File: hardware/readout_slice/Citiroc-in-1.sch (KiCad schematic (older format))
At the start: 6 parts

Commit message: need to fix one rescure in readout_slice
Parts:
- U?: symbol readout_slice-rescue:CITIROC1A-readout -> readout_slice-rescue:CITIROC1A-readout-readout_slice-rescue
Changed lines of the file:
@@
 $Descr A4 11693 8268
 encoding utf-8
-Sheet 7 16
+Sheet 6 16
 Title ""
 Date ""
@@
 	9450 1600 3800 1600
 $Comp
-L readout_slice-rescue:CITIROC1A-readout U?
+L readout_slice-rescue:CITIROC1A-readout-readout_slice-rescue U?
 U 3 1 60AFA4EB
 P 10100 900

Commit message: getting rid of readout_slice rescue
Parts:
- U?: symbol readout_slice-rescue:CITIROC1A-readout-readout_slice-rescue -> readout:CITIROC1A
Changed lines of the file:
@@
 	9450 1600 3800 1600
 $Comp
-L readout_slice-rescue:CITIROC1A-readout-readout_slice-rescue U?
+L readout:CITIROC1A U?
 U 3 1 60AFA4EB
 P 10100 900

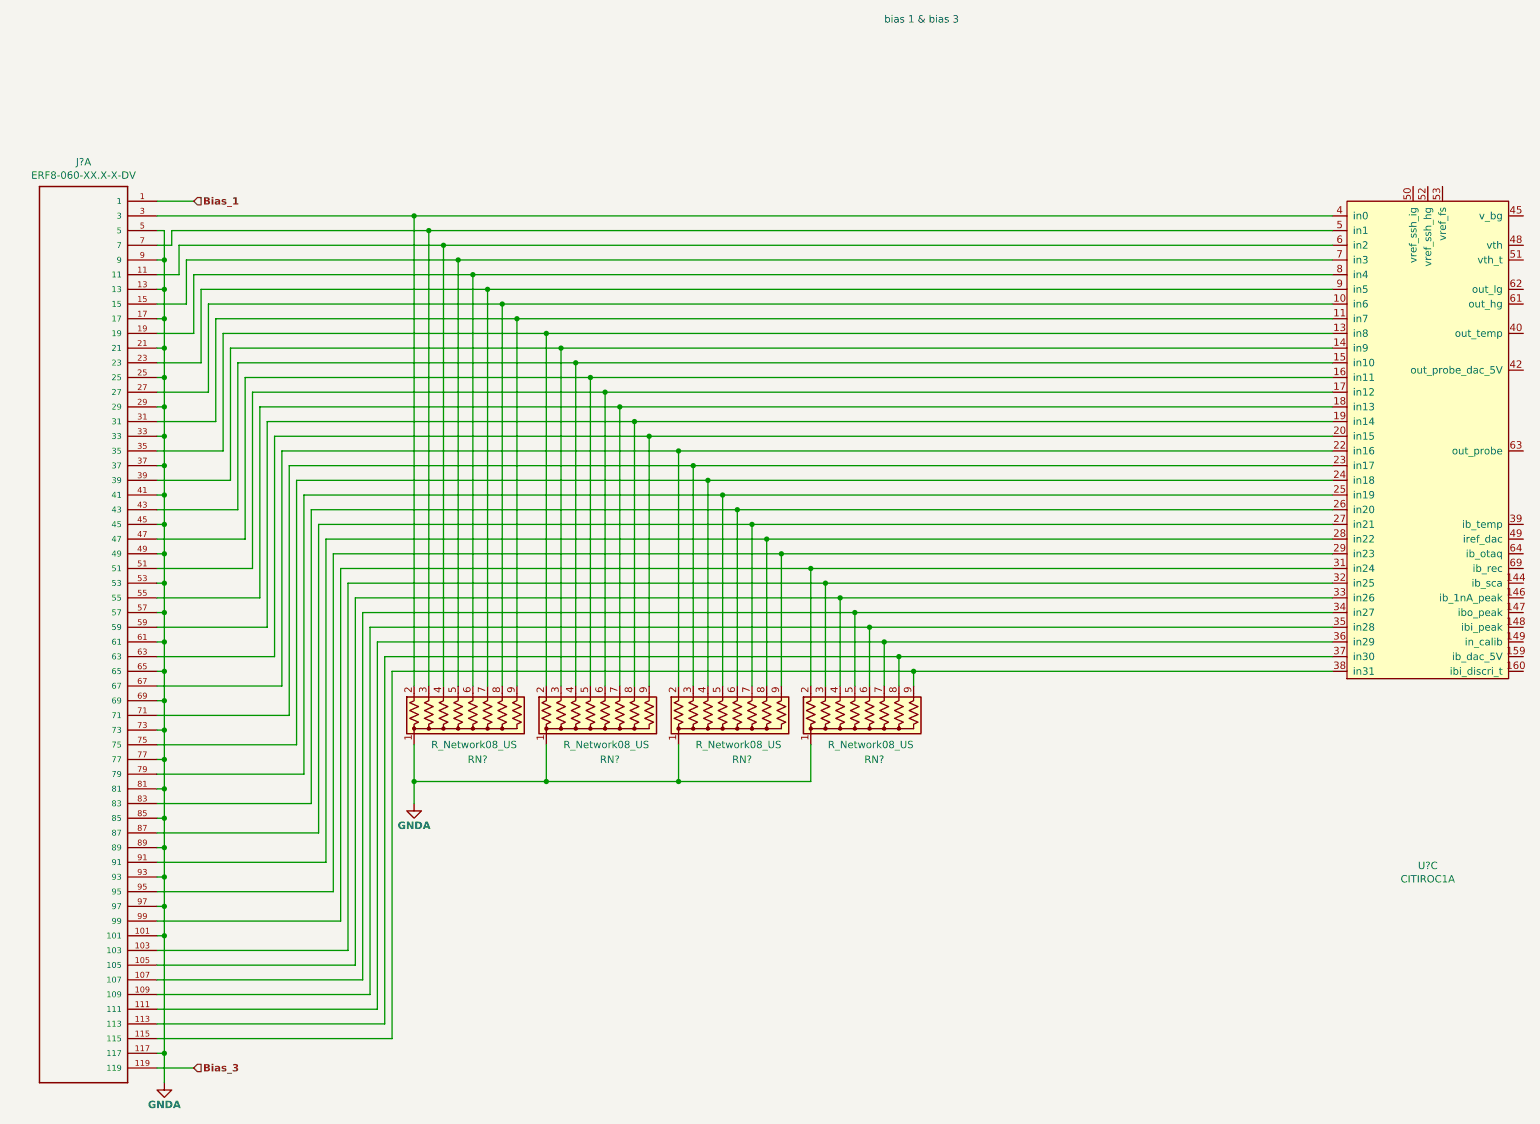
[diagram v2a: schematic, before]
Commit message: more progress on readout_slice
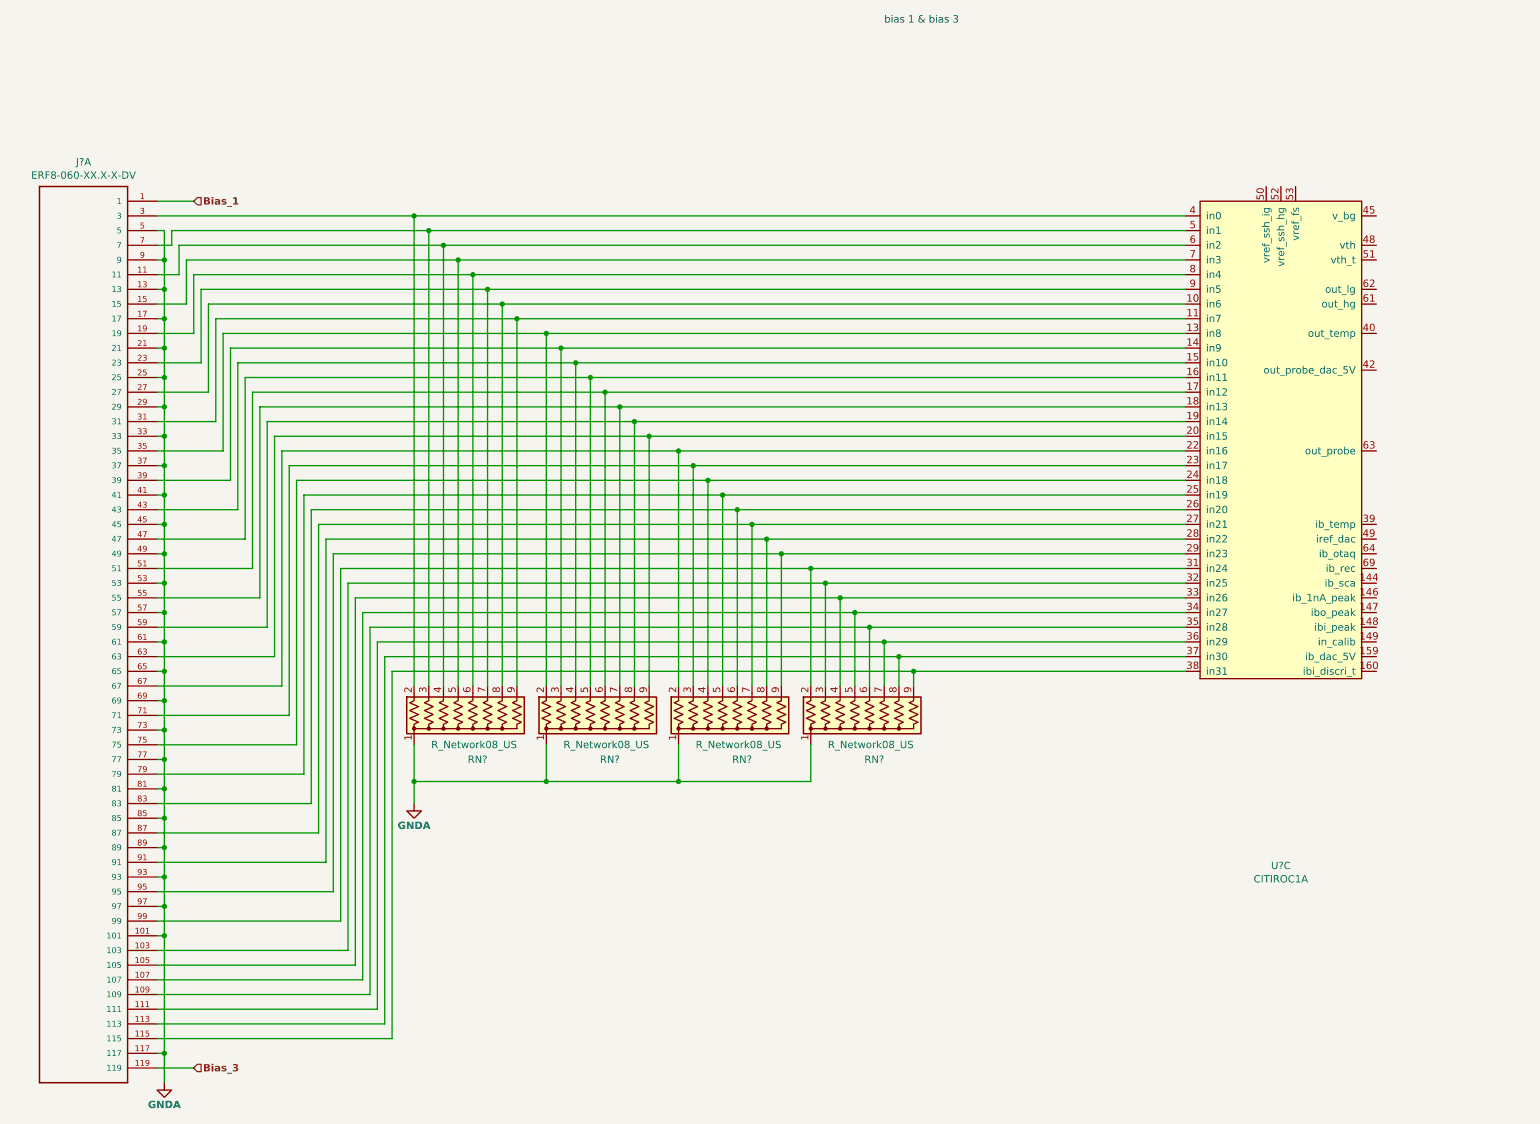
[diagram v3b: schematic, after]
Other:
- moved on the sheet: U?C
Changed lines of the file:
@@
 	1700 6800 1450 6800
 Wire Wire Line
-	3700 1500 9450 1500
+	3700 1500 8450 1500
 Wire Wire Line
-	9450 1400 3600 1400
+	8450 1400 3600 1400
 Wire Wire Line
-	3500 1300 9450 1300
+	3500 1300 8450 1300
 Wire Wire Line
-	9450 1200 3400 1200
+	8450 1200 3400 1200
 Wire Wire Line
-	3300 1100 9450 1100
+	3300 1100 8450 1100
 Wire Wire Line
-	9450 1000 3200 1000
+	8450 1000 3200 1000
 Wire Wire Line
-	6600 4100 9450 4100
+	6600 4100 8450 4100
 Wire Wire Line
-	6500 4000 9450 4000
+	6500 4000 8450 4000
 Wire Wire Line
-	6400 3900 9450 3900
+	6400 3900 8450 3900
 Wire Wire Line
-	6300 3800 9450 3800
+	6300 3800 8450 3800
 Wire Wire Line
-	6200 3700 9450 3700
+	6200 3700 8450 3700
 Wire Wire Line
-	9450 3600 6100 3600
+	8450 3600 6100 3600
 Wire Wire Line
-	9450 3500 6000 3500
+	8450 3500 6000 3500
 Wire Wire Line
-	5900 3400 9450 3400
+	5900 3400 8450 3400
 Wire Wire Line
-	9450 3300 5700 3300
+	8450 3300 5700 3300
 Wire Wire Line
-	5600 3200 9450 3200
+	5600 3200 8450 3200
 Wire Wire Line
-	9450 3100 5500 3100
+	8450 3100 5500 3100
 Wire Wire Line
-	5400 3000 9450 3000
+	5400 3000 8450 3000
 Wire Wire Line
-	9450 2900 5300 2900
+	8450 2900 5300 2900
 Wire Wire Line
-	5200 2800 9450 2800
+	5200 2800 8450 2800
 Wire Wire Line
-	9450 2700 5100 2700
+	8450 2700 5100 2700
 Wire Wire Line
-	5000 2600 9450 2600
+	5000 2600 8450 2600
 Wire Wire Line
-	9450 2500 4800 2500
+	8450 2500 4800 2500
 Wire Wire Line
-	4700 2400 9450 2400
+	4700 2400 8450 2400
 Wire Wire Line
-	9450 2300 4600 2300
+	8450 2300 4600 2300
 Wire Wire Line
-	4500 2200 9450 2200
+	4500 2200 8450 2200
 Wire Wire Line
-	9450 2100 4400 2100
+	8450 2100 4400 2100
 Wire Wire Line
-	4300 2000 9450 2000
+	4300 2000 8450 2000
 Wire Wire Line
-	9450 1900 4200 1900
+	8450 1900 4200 1900
 Wire Wire Line
-	4100 1800 9450 1800
+	4100 1800 8450 1800
 Wire Wire Line
-	3900 1700 9450 1700
+	3900 1700 8450 1700
 Wire Wire Line
-	9450 1600 3800 1600
+	8450 1600 3800 1600
 $Comp
 L readout:CITIROC1A U?
 U 3 1 60AFA4EB
-P 10100 900
+P 9100 900
 AR Path="/60AFA4EB" Ref="U?"  Part="3"
 AR Path="/6076454A/60AFA4EB" Ref="U?"  Part="3"
-F 0 "U?" H 10100 -3623 50  0000 C CNN
-F 1 "CITIROC1A" H 10100 -3714 50  0000 C CNN
-F 2 "Package_QFP:LQFP-160_24x24mm_P0.5mm" H 9500 1050 50  0001 C CNN
-F 3 "http://gauss.bu.edu/svn/emphatic-doco/Docs/CITIROC1A%20-%20Datasheet%20V2.5.pdf" H 9500 1050 50  0001 C CNN
-	3    10100 900
+F 0 "U?" H 9100 -3623 50  0000 C CNN
+F 1 "CITIROC1A" H 9100 -3714 50  0000 C CNN
+F 2 "Package_QFP:LQFP-160_24x24mm_P0.5mm" H 8500 1050 50  0001 C CNN
+F 3 "http://gauss.bu.edu/svn/emphatic-doco/Docs/CITIROC1A%20-%20Datasheet%20V2.5.pdf" H 8500 1050 50  0001 C CNN
+	3    9100 900
 	1    0    0    -1
 $EndComp
